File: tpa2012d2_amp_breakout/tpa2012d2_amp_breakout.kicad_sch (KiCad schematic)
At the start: 4 parts, among them J101 Conn_01x07_Female, J102 SPK L, J103 SPK R, J104 AudioJack3

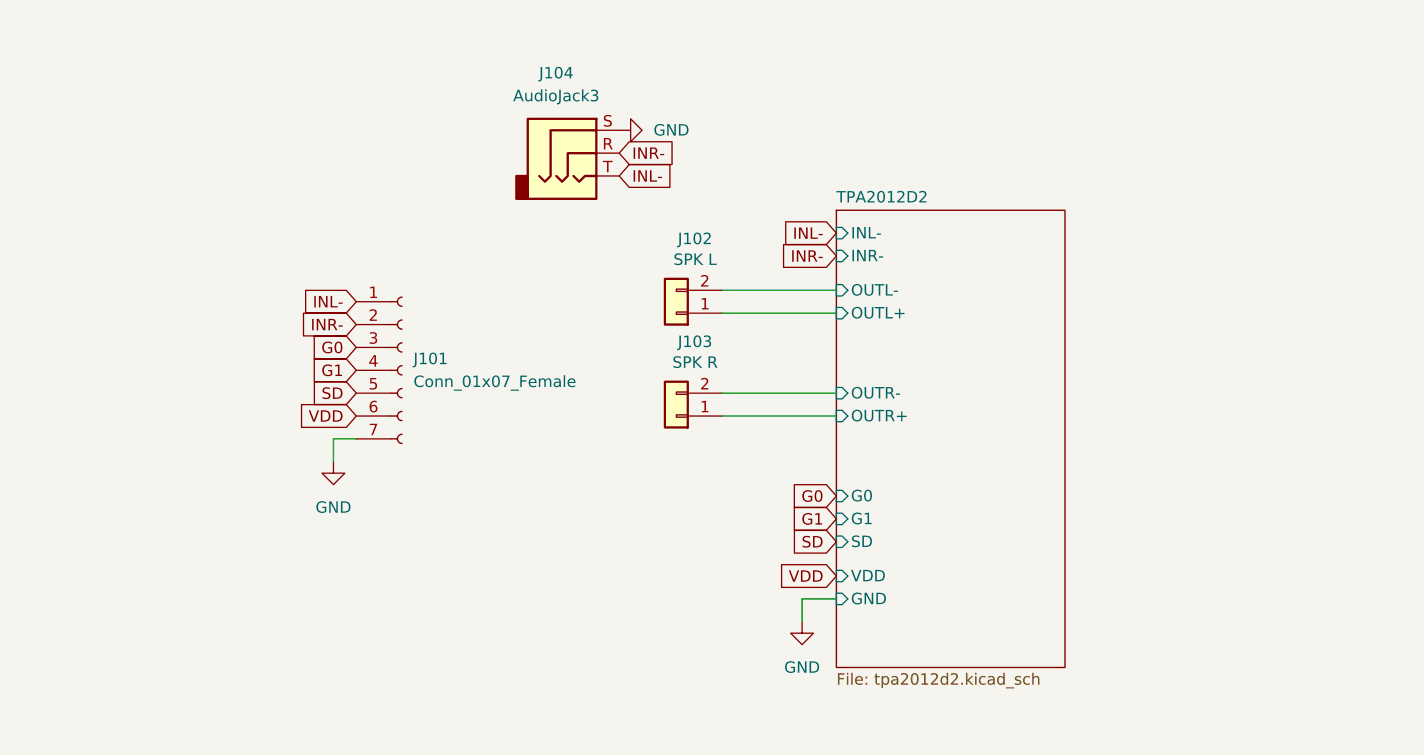
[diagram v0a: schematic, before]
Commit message: WIP
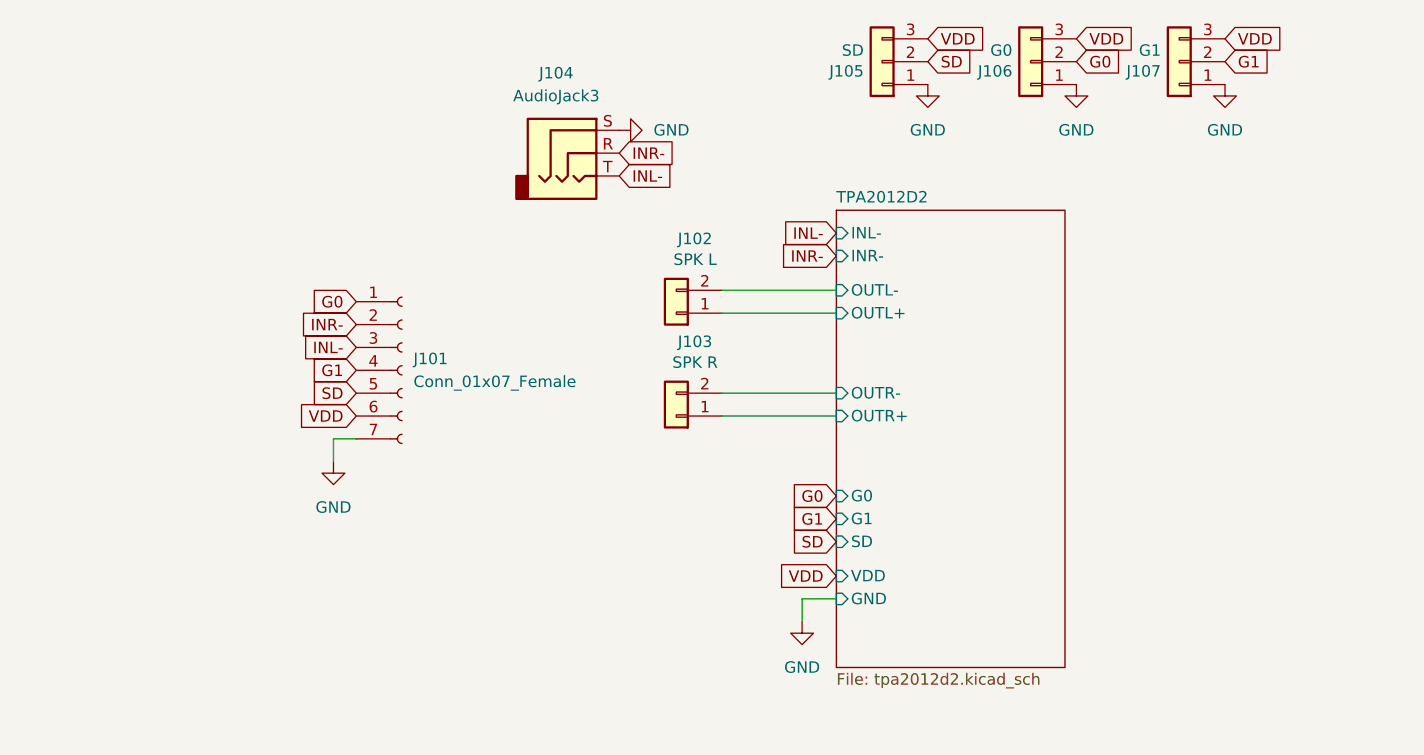
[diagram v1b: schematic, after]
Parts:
- added J105: SD, Connector_PinHeader_2.54mm:PinHeader_1x03_P2.54mm_Vertical, symbol Connector_Generic:Conn_01x03
- added J106: G0, Connector_PinHeader_2.54mm:PinHeader_1x03_P2.54mm_Vertical, symbol Connector_Generic:Conn_01x03
- added J107: G1, Connector_PinHeader_2.54mm:PinHeader_1x03_P2.54mm_Vertical, symbol Connector_Generic:Conn_01x03
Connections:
- net G0: now also J101.1 (Pin_1), J106.2 (Pin_2); no longer J101.3 (Pin_3)
- net G1: now also J107.2 (Pin_2)
- net GND: now also J105.1 (Pin_1), J106.1 (Pin_1), J107.1 (Pin_1)
- net INL-: now also J101.3 (Pin_3); no longer J101.1 (Pin_1)
- net SD: now also J105.2 (Pin_2)
- net VDD: now also J105.3 (Pin_3), J106.3 (Pin_3), J107.3 (Pin_3)
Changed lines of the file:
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@@
     (stroke (width 0) (type default) (color 0 0 0 0))
   )
-  (global_label "G0" (shape input) (at 116.84 92.71 180) (fields_autoplaced)
-    (effects (font (size 1.27 1.27)) (justify right))
-    (property "Intersheet References" "${INTERSHEET_REFS}" (id 0) (at 111.9474 92.6306 0)
-      (effects (font (size 1.27 1.27)) (justify right) hide)
+  (global_label "G0" (shape input) (at 116.84 87.63 180) (fields_autoplaced)
+    (effects (font (size 1.27 1.27)) (justify right))
+    (property "Intersheet References" "${INTERSHEET_REFS}" (id 0) (at 111.9474 87.5506 0)
+      (effects (font (size 1.27 1.27)) (justify right) hide)
+    )
+  )
+  (global_label "G1" (shape input) (at 213.36 60.96 0) (fields_autoplaced)
+    (effects (font (size 1.27 1.27)) (justify left))
+    (property "Intersheet References" "${INTERSHEET_REFS}" (id 0) (at 218.2526 61.0394 0)
+      (effects (font (size 1.27 1.27)) (justify left) hide)
     )
   )
@@
     )
   )
-  (global_label "INL-" (shape input) (at 116.84 87.63 180) (fields_autoplaced)
-    (effects (font (size 1.27 1.27)) (justify right))
-    (property "Intersheet References" "${INTERSHEET_REFS}" (id 0) (at 109.8912 87.5506 0)
-      (effects (font (size 1.27 1.27)) (justify right) hide)
+  (global_label "VDD" (shape input) (at 180.34 58.42 0) (fields_autoplaced)
+    (effects (font (size 1.27 1.27)) (justify left))
+    (property "Intersheet References" "${INTERSHEET_REFS}" (id 0) (at 186.3817 58.4994 0)
+      (effects (font (size 1.27 1.27)) (justify left) hide)
+    )
+  )
+  (global_label "INL-" (shape input) (at 116.84 92.71 180) (fields_autoplaced)
+    (effects (font (size 1.27 1.27)) (justify right))
+    (property "Intersheet References" "${INTERSHEET_REFS}" (id 0) (at 109.8912 92.6306 0)
+      (effects (font (size 1.27 1.27)) (justify right) hide)
+    )
+  )
+  (global_label "G0" (shape input) (at 196.85 60.96 0) (fields_autoplaced)
+    (effects (font (size 1.27 1.27)) (justify left))
+    (property "Intersheet References" "${INTERSHEET_REFS}" (id 0) (at 201.7426 61.0394 0)
+      (effects (font (size 1.27 1.27)) (justify left) hide)
     )
   )
@@
     )
   )
+  (global_label "VDD" (shape input) (at 196.85 58.42 0) (fields_autoplaced)
+    (effects (font (size 1.27 1.27)) (justify left))
+    (property "Intersheet References" "${INTERSHEET_REFS}" (id 0) (at 202.8917 58.4994 0)
+      (effects (font (size 1.27 1.27)) (justify left) hide)
+    )
+  )
+  (global_label "VDD" (shape input) (at 213.36 58.42 0) (fields_autoplaced)
+    (effects (font (size 1.27 1.27)) (justify left))
+    (property "Intersheet References" "${INTERSHEET_REFS}" (id 0) (at 219.4017 58.4994 0)
+      (effects (font (size 1.27 1.27)) (justify left) hide)
+    )
+  )
   (global_label "G1" (shape input) (at 170.18 111.76 180) (fields_autoplaced)
     (effects (font (size 1.27 1.27)) (justify right))
@@
       (effects (font (size 1.27 1.27)) (justify right) hide)
     )
+  )
+  (global_label "SD" (shape input) (at 180.34 60.96 0) (fields_autoplaced)
+    (effects (font (size 1.27 1.27)) (justify left))
+    (property "Intersheet References" "${INTERSHEET_REFS}" (id 0) (at 185.2326 61.0394 0)
+      (effects (font (size 1.27 1.27)) (justify left) hide)
+    )
+  )
+  (symbol (lib_id "power:GND") (at 180.34 63.5 0) (unit 1)
+    (in_bom yes) (on_board yes) (fields_autoplaced)
+    (property "Reference" "#PWR0106" (id 0) (at 180.34 69.85 0)
+      (effects (font (size 1.27 1.27)) hide)
+    )
+    (property "Value" "GND" (id 1) (at 180.34 68.58 0))
+    (property "Footprint" "" (id 2) (at 180.34 63.5 0)
+      (effects (font (size 1.27 1.27)) hide)
+    )
+    (property "Datasheet" "" (id 3) (at 180.34 63.5 0)
+      (effects (font (size 1.27 1.27)) hide)
+    )
+    (pin "1")
   )
   (symbol (lib_id "Connector_Generic:Conn_01x02") (at 152.4 100.33 180) (unit 1)
@@
     (pin "1")
   )
+  (symbol (lib_id "power:GND") (at 213.36 63.5 0) (unit 1)
+    (in_bom yes) (on_board yes) (fields_autoplaced)
+    (property "Reference" "#PWR0105" (id 0) (at 213.36 69.85 0)
+      (effects (font (size 1.27 1.27)) hide)
+    )
+    (property "Value" "GND" (id 1) (at 213.36 68.58 0))
+    (property "Footprint" "" (id 2) (at 213.36 63.5 0)
+      (effects (font (size 1.27 1.27)) hide)
+    )
+    (property "Datasheet" "" (id 3) (at 213.36 63.5 0)
+      (effects (font (size 1.27 1.27)) hide)
+    )
+    (pin "1")
+  )
+  (symbol (lib_id "power:GND") (at 196.85 63.5 0) (unit 1)
+    (in_bom yes) (on_board yes) (fields_autoplaced)
+    (property "Reference" "#PWR0104" (id 0) (at 196.85 69.85 0)
+      (effects (font (size 1.27 1.27)) hide)
+    )
+    (property "Value" "GND" (id 1) (at 196.85 68.58 0))
+    (property "Footprint" "" (id 2) (at 196.85 63.5 0)
+      (effects (font (size 1.27 1.27)) hide)
+    )
+    (property "Datasheet" "" (id 3) (at 196.85 63.5 0)
+      (effects (font (size 1.27 1.27)) hide)
+    )
+    (pin "1")
+  )
   (symbol (lib_id "power:GND") (at 114.3 105.41 0) (unit 1)
     (in_bom yes) (on_board yes) (fields_autoplaced)
@@
     (pin "2")
   )
+  (symbol (lib_id "Connector_Generic:Conn_01x03") (at 191.77 60.96 180) (unit 1)
+    (in_bom yes) (on_board yes)
+    (property "Reference" "J106" (id 0) (at 189.738 62.0268 0)
+      (effects (font (size 1.27 1.27)) (justify left))
+    )
+    (property "Value" "G0" (id 1) (at 189.738 59.7154 0)
+      (effects (font (size 1.27 1.27)) (justify left))
+    )
+    (property "Footprint" "Connector_PinHeader_2.54mm:PinHeader_1x03_P2.54mm_Vertical" (id 2) (at 191.77 60.96 0)
+      (effects (font (size 1.27 1.27)) hide)
+    )
+    (property "Datasheet" "~" (id 3) (at 191.77 60.96 0)
+      (effects (font (size 1.27 1.27)) hide)
+    )
+    (property "JLCPCB BOM" "False" (id 4) (at 191.77 60.96 0)
+      (effects (font (size 1.27 1.27)) hide)
+    )
+    (pin "1")
+    (pin "2")
+    (pin "3")
+  )
+  (symbol (lib_id "Connector_Generic:Conn_01x03") (at 208.28 60.96 180) (unit 1)
+    (in_bom yes) (on_board yes)
+    (property "Reference" "J107" (id 0) (at 206.248 62.0268 0)
+      (effects (font (size 1.27 1.27)) (justify left))
+    )
+    (property "Value" "G1" (id 1) (at 206.248 59.7154 0)
+      (effects (font (size 1.27 1.27)) (justify left))
+    )
+    (property "Footprint" "Connector_PinHeader_2.54mm:PinHeader_1x03_P2.54mm_Vertical" (id 2) (at 208.28 60.96 0)
+      (effects (font (size 1.27 1.27)) hide)
+    )
+    (property "Datasheet" "~" (id 3) (at 208.28 60.96 0)
+      (effects (font (size 1.27 1.27)) hide)
+    )
+    (property "JLCPCB BOM" "False" (id 4) (at 208.28 60.96 0)
+      (effects (font (size 1.27 1.27)) hide)
+    )
+    (pin "1")
+    (pin "2")
+    (pin "3")
+  )
+  (symbol (lib_id "Connector_Generic:Conn_01x03") (at 175.26 60.96 180) (unit 1)
+    (in_bom yes) (on_board yes)
+    (property "Reference" "J105" (id 0) (at 173.228 62.0268 0)
+      (effects (font (size 1.27 1.27)) (justify left))
+    )
+    (property "Value" "SD" (id 1) (at 173.228 59.7154 0)
+      (effects (font (size 1.27 1.27)) (justify left))
+    )
+    (property "Footprint" "Connector_PinHeader_2.54mm:PinHeader_1x03_P2.54mm_Vertical" (id 2) (at 175.26 60.96 0)
+      (effects (font (size 1.27 1.27)) hide)
+    )
+    (property "Datasheet" "~" (id 3) (at 175.26 60.96 0)
+      (effects (font (size 1.27 1.27)) hide)
+    )
+    (property "JLCPCB BOM" "False" (id 4) (at 175.26 60.96 0)
+      (effects (font (size 1.27 1.27)) hide)
+    )
+    (pin "1")
+    (pin "2")
+    (pin "3")
+  )
   (sheet (at 170.18 77.47) (size 25.4 50.8) (fields_autoplaced)
     (stroke (width 0.1524) (type solid) (color 0 0 0 0))
@@
       (reference "#PWR0103") (unit 1) (value "GND") (footprint "")
     )
+    (path "/07f0eb42-5932-4c16-9d2f-e1b13871baff"
+      (reference "#PWR0104") (unit 1) (value "GND") (footprint "")
+    )
+    (path "/06968dfa-a45e-4c85-80a1-b3e78c7cf0f9"
+      (reference "#PWR0105") (unit 1) (value "GND") (footprint "")
+    )
+    (path "/01de6145-2e02-4aeb-8134-a8ad1f76eb95"
+      (reference "#PWR0106") (unit 1) (value "GND") (footprint "")
+    )
     (path "/245afab8-87c2-4797-af78-aa00d5229c94/4f81fe66-376f-435c-bded-ecdb05d77dd8"
       (reference "C301") (unit 1) (value "1u") (footprint "Capacitor_SMD:C_0603_1608Metric")
@@
       (reference "J104") (unit 1) (value "AudioJack3") (footprint "tpa2012d2:PJ-320B-3A")
     )
+    (path "/ee737e09-c622-45af-bfe6-b2882f4c573f"
+      (reference "J105") (unit 1) (value "SD") (footprint "Connector_PinHeader_2.54mm:PinHeader_1x03_P2.54mm_Vertical")
+    )
+    (path "/b6977247-0e8e-422f-b397-a64eed1d46da"
+      (reference "J106") (unit 1) (value "G0") (footprint "Connector_PinHeader_2.54mm:PinHeader_1x03_P2.54mm_Vertical")
+    )
+    (path "/d599ee5f-5c96-4c6d-a4f2-87e98db0087b"
+      (reference "J107") (unit 1) (value "G1") (footprint "Connector_PinHeader_2.54mm:PinHeader_1x03_P2.54mm_Vertical")
+    )
     (path "/245afab8-87c2-4797-af78-aa00d5229c94/0d6e844c-e4e3-4bae-99c1-0281f5127920"

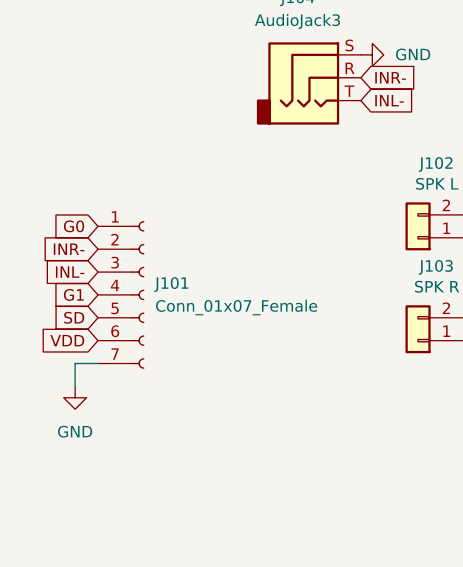
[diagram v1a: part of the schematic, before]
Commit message: WIP
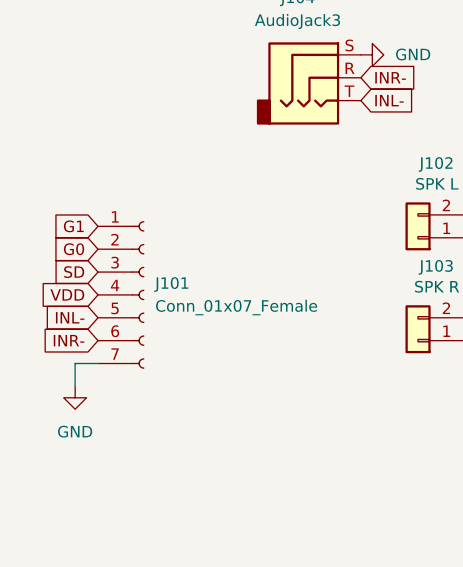
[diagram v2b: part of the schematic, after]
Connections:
- net G0: now also J101.2 (Pin_2); no longer J101.1 (Pin_1)
- net G1: now also J101.1 (Pin_1); no longer J101.4 (Pin_4)
- net INL-: now also J101.5 (Pin_5); no longer J101.3 (Pin_3)
- net INR-: now also J101.6 (Pin_6); no longer J101.2 (Pin_2)
- net SD: now also J101.3 (Pin_3); no longer J101.5 (Pin_5)
- net VDD: now also J101.4 (Pin_4); no longer J101.6 (Pin_6)
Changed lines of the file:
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@@
     (stroke (width 0) (type default) (color 0 0 0 0))
   )
-  (global_label "G0" (shape input) (at 116.84 87.63 180) (fields_autoplaced)
+  (global_label "G0" (shape input) (at 116.84 90.17 180) (fields_autoplaced)
     (effects (font (size 1.27 1.27)) (justify right))
-    (property "Intersheet References" "${INTERSHEET_REFS}" (id 0) (at 111.9474 87.5506 0)
+    (property "Intersheet References" "${INTERSHEET_REFS}" (id 0) (at 111.9474 90.0906 0)
       (effects (font (size 1.27 1.27)) (justify right) hide)
     )
@@
     )
   )
-  (global_label "G1" (shape input) (at 116.84 95.25 180) (fields_autoplaced)
+  (global_label "G1" (shape input) (at 116.84 87.63 180) (fields_autoplaced)
     (effects (font (size 1.27 1.27)) (justify right))
-    (property "Intersheet References" "${INTERSHEET_REFS}" (id 0) (at 111.9474 95.1706 0)
+    (property "Intersheet References" "${INTERSHEET_REFS}" (id 0) (at 111.9474 87.5506 0)
       (effects (font (size 1.27 1.27)) (justify right) hide)
     )
   )
-  (global_label "VDD" (shape input) (at 116.84 100.33 180) (fields_autoplaced)
+  (global_label "VDD" (shape input) (at 116.84 95.25 180) (fields_autoplaced)
     (effects (font (size 1.27 1.27)) (justify right))
-    (property "Intersheet References" "${INTERSHEET_REFS}" (id 0) (at 110.7983 100.2506 0)
+    (property "Intersheet References" "${INTERSHEET_REFS}" (id 0) (at 110.7983 95.1706 0)
       (effects (font (size 1.27 1.27)) (justify right) hide)
     )
@@
     )
   )
-  (global_label "INL-" (shape input) (at 116.84 92.71 180) (fields_autoplaced)
+  (global_label "INL-" (shape input) (at 116.84 97.79 180) (fields_autoplaced)
     (effects (font (size 1.27 1.27)) (justify right))
-    (property "Intersheet References" "${INTERSHEET_REFS}" (id 0) (at 109.8912 92.6306 0)
+    (property "Intersheet References" "${INTERSHEET_REFS}" (id 0) (at 109.8912 97.7106 0)
       (effects (font (size 1.27 1.27)) (justify right) hide)
     )
@@
     )
   )
-  (global_label "SD" (shape input) (at 116.84 97.79 180) (fields_autoplaced)
+  (global_label "SD" (shape input) (at 116.84 92.71 180) (fields_autoplaced)
     (effects (font (size 1.27 1.27)) (justify right))
-    (property "Intersheet References" "${INTERSHEET_REFS}" (id 0) (at 111.9474 97.7106 0)
+    (property "Intersheet References" "${INTERSHEET_REFS}" (id 0) (at 111.9474 92.6306 0)
       (effects (font (size 1.27 1.27)) (justify right) hide)
     )
@@
     )
   )
-  (global_label "INR-" (shape input) (at 116.84 90.17 180) (fields_autoplaced)
+  (global_label "INR-" (shape input) (at 116.84 100.33 180) (fields_autoplaced)
     (effects (font (size 1.27 1.27)) (justify right))
-    (property "Intersheet References" "${INTERSHEET_REFS}" (id 0) (at 109.6493 90.0906 0)
+    (property "Intersheet References" "${INTERSHEET_REFS}" (id 0) (at 109.6493 100.2506 0)
       (effects (font (size 1.27 1.27)) (justify right) hide)
     )
